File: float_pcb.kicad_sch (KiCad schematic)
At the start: 55 parts, among them J1 Switch, J2 Conn_01x04, J3 USB_C, J4 Conn_01x03, J5 I2C, J6 Light, J7 Batt, J9 I2C, Q1 AO3400A, Q2 AO3400A, U1 TPSM863252, U2 TPSM863252, U4 ESP32-S3-WROOM-1

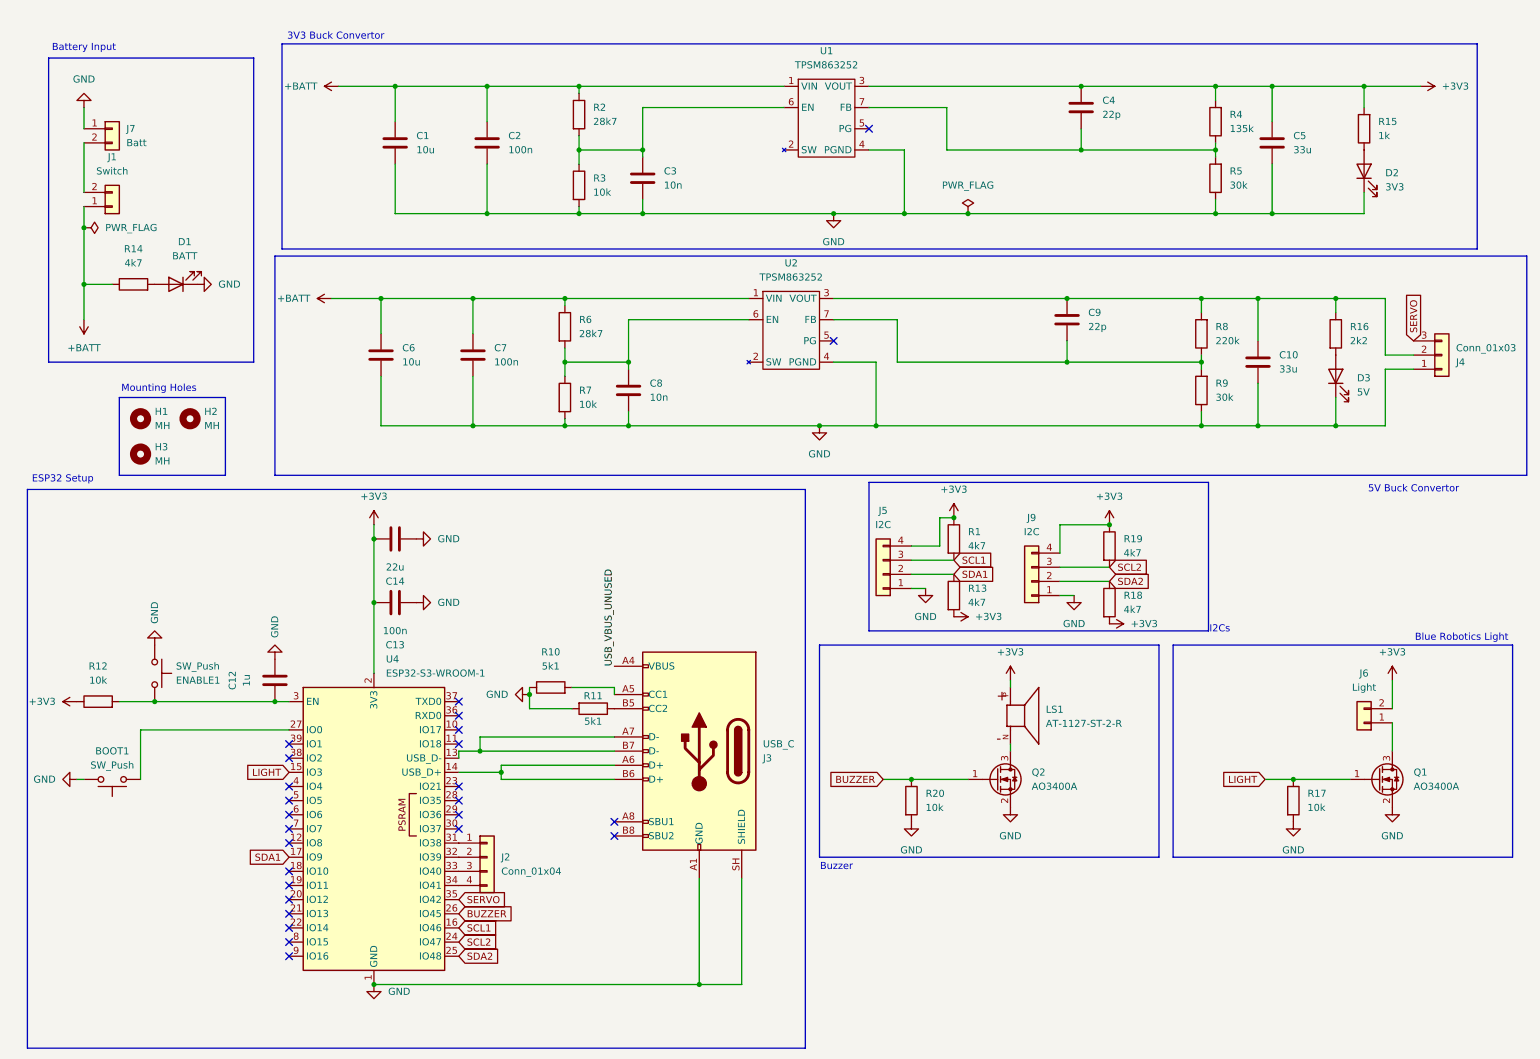
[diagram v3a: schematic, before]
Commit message: Version 3
Before the big 4 layer migration
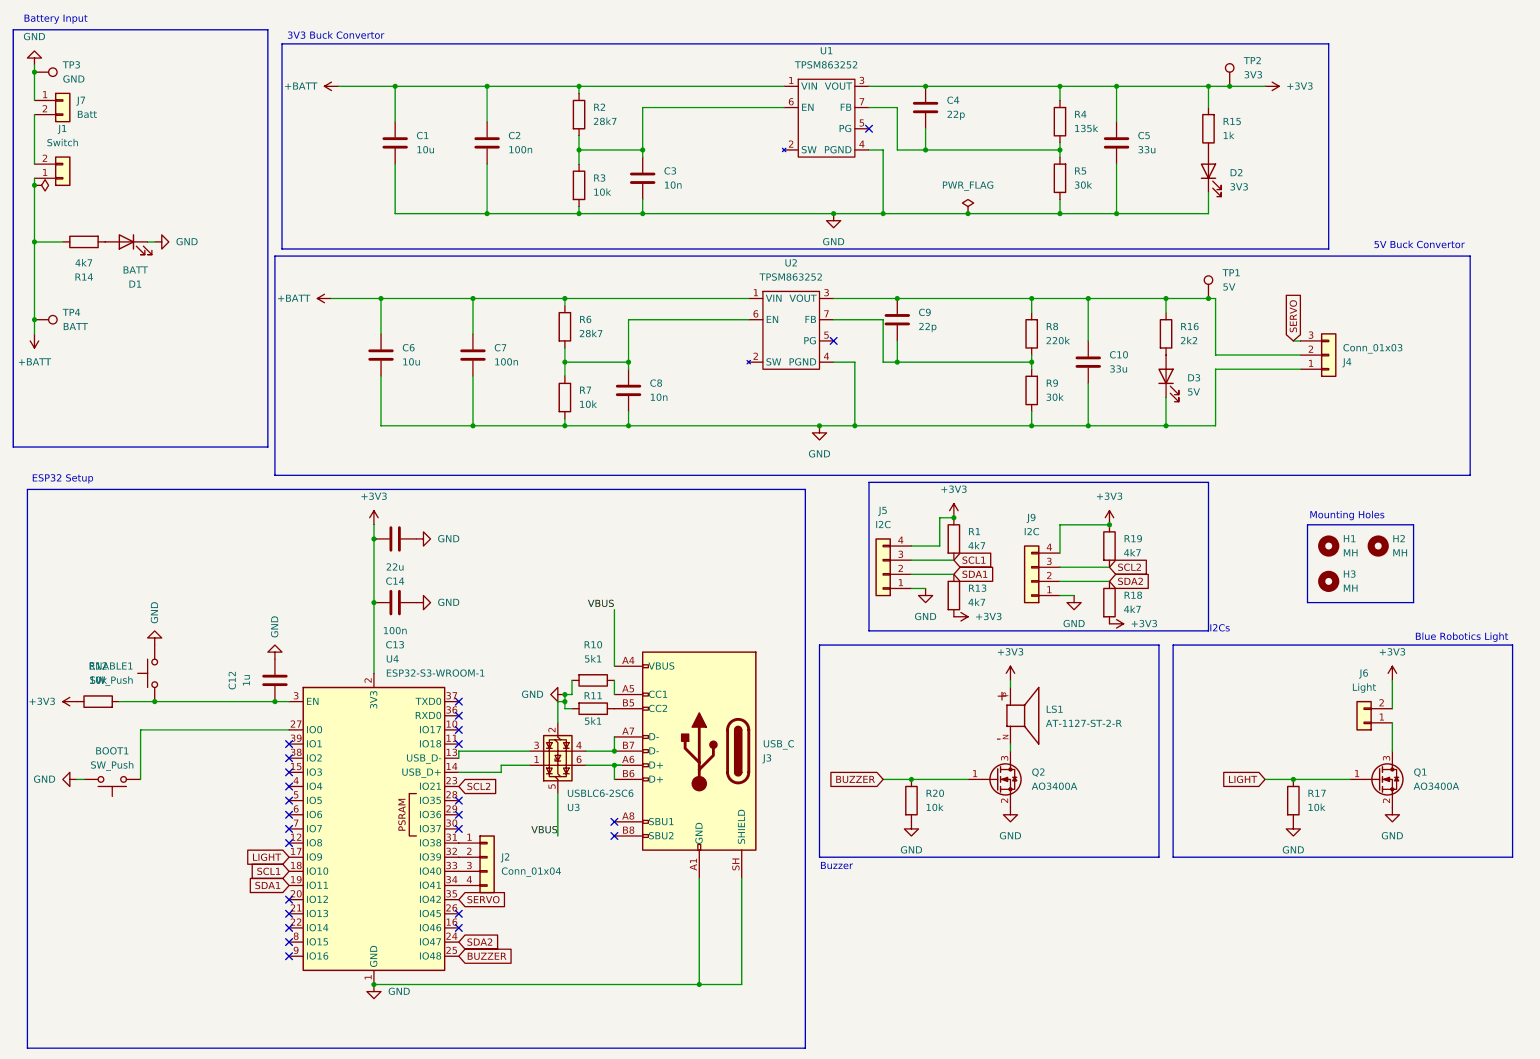
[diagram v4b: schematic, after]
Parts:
- added TP1: 5V, TestPoint:TestPoint_Pad_D1.5mm, symbol Connector:TestPoint
- added TP2: 3V3, TestPoint:TestPoint_Pad_D1.5mm, symbol Connector:TestPoint
- added TP3: GND, TestPoint:TestPoint_Pad_D1.5mm, symbol Connector:TestPoint
- added TP4: BATT, TestPoint:TestPoint_Pad_D1.5mm, symbol Connector:TestPoint
- added U3: USBLC6-2SC6, Package_TO_SOT_SMD:SOT-23-6, symbol Power_Protection:USBLC6-2SC6
- C1, C10, C5, C6: footprint Capacitor_SMD:C_0603_1608Metric -> Capacitor_SMD:C_0805_2012Metric
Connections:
- net +3V3: now also C4.1, TP2.1; no longer C4.2
- net +BATT: now also C1.1, C2.2, TP4.1; no longer C1.2, C2.1
- net BUZZER: now also U4.25 (IO48); no longer U4.26 (IO45)
- net GND: now also C1.2, C2.1, C3.1, ENABLE1.2, R10.2, TP3.1, U3.2 (GND); no longer C1.1, C2.2, C3.2, ENABLE1.1, R10.1
- net LIGHT: now also U4.17 (IO9); no longer U4.15 (IO3)
- net SCL1: now also U4.18 (IO10); no longer U4.16 (IO46)
- net SCL2: now also U4.23 (IO21); no longer U4.24 (IO47)
- net SDA1: now also U4.19 (IO11); no longer U4.17 (IO9)
- net SDA2: now also U4.24 (IO47); no longer U4.25 (IO48)
- net at R8.1, R9.2, U2.7 (FB): now also C9.2; no longer C9.1
- net at C10.2, J4.2 (Pin_2), R16.1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: now also C9.1, TP1.1; no longer C9.2
- net at R2.2, R3.1, U1.6 (EN): now also C3.2; no longer C3.1
- net at R4.1, R5.2, U1.7 (FB): now also C4.2; no longer C4.1
- net at C12.2, R12.2, U4.3 (EN): now also ENABLE1.1; no longer ENABLE1.2
- net at J3.A5 (CC1): now also R10.1; no longer R10.2
- net at J3.A6 (D+), J3.B6 (D+): now also U3.6 (I/O1); no longer U4.14 (USB_D+)
- net at J3.A7 (D-), J3.B7 (D-): now also U3.4 (I/O2); no longer U4.13 (USB_D-)
- net USB_VBUS_UNUSED renamed VBUS
- net VBUS: now also U3.5 (VBUS)
- new net: U3.3 (I/O2), U4.13 (USB_D-)
- new net: U3.1 (I/O1), U4.14 (USB_D+)
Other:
- company: Leviathan Underwater Robotics -> Leviathan Underwater Robotics (Evan Kim)
- moved on the sheet: C1, C10, C2, C3, C4, C5, C9, D1, D2, D3, ENABLE1, H1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
